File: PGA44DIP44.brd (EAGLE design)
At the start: 58.1 x 20.3 mm, 6 parts

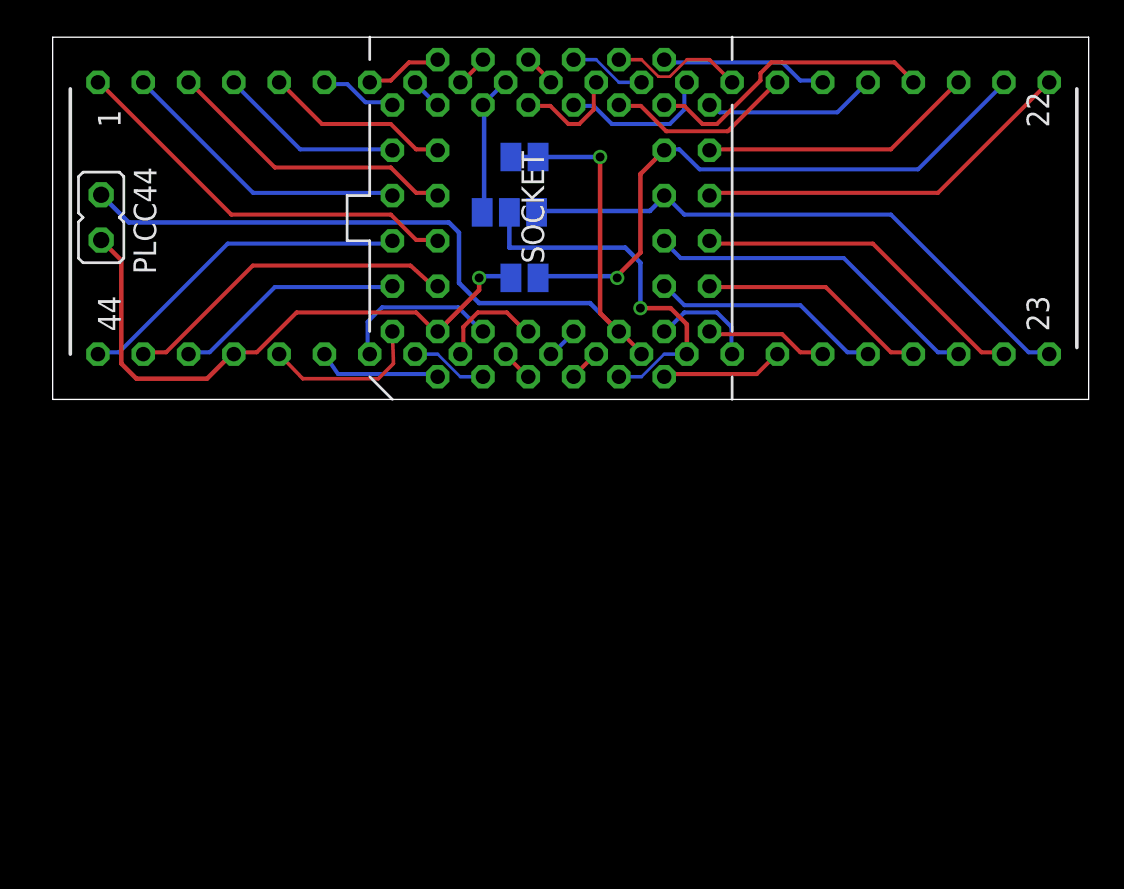
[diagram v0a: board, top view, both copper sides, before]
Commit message: Move to origin.
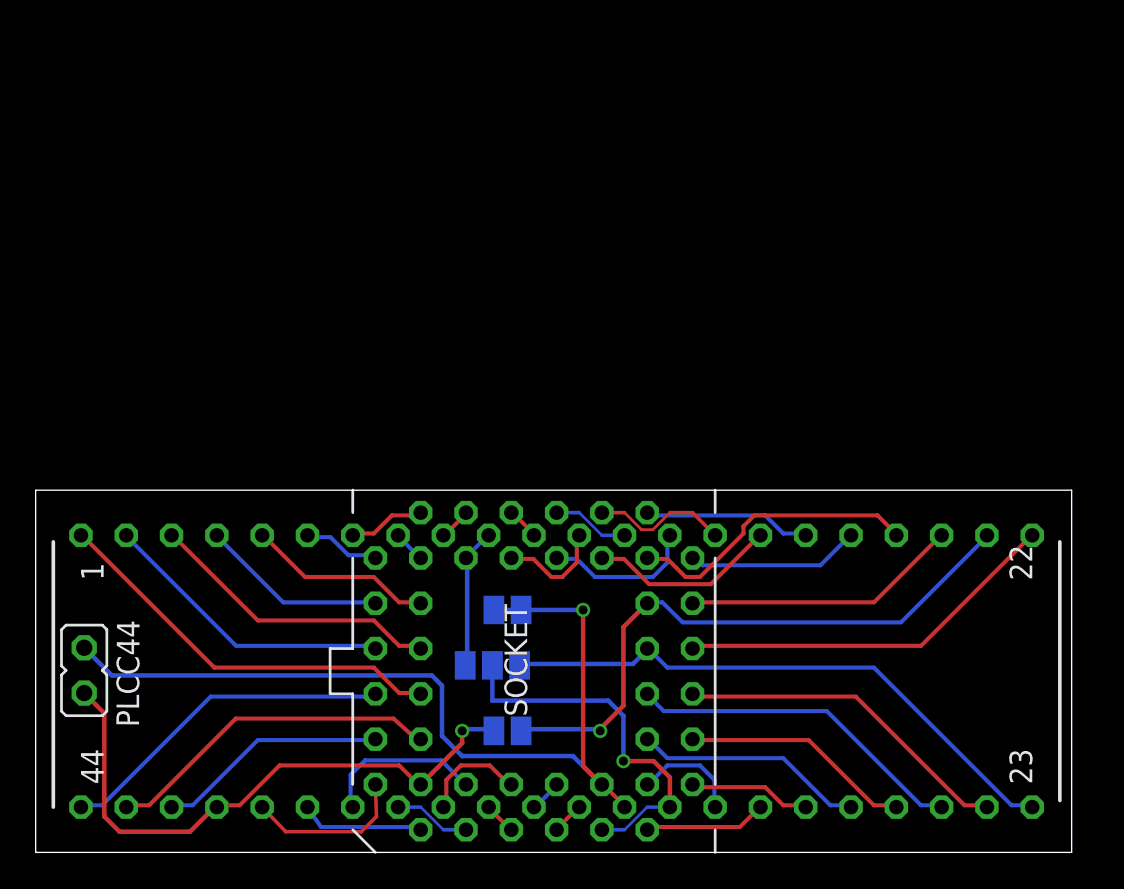
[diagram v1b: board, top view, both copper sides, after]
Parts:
- moved SOCKET 25.4 mm to (27.9, 10.2)
- moved 　　　 25.4 mm to (25.6, 10.5)
- moved 　　　　 25.4 mm to (26.5, 13.6)
- moved 　 25.4 mm to (2.72, 10.2)
- moved PLCC44 25.4 mm to (29.2, 11.4)
- moved 　　 25.4 mm to (26.5, 6.81)
